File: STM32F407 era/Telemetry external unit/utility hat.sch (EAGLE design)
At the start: 4 parts, among them U1 SC18IM700IPW,112, U2 MAX1704X

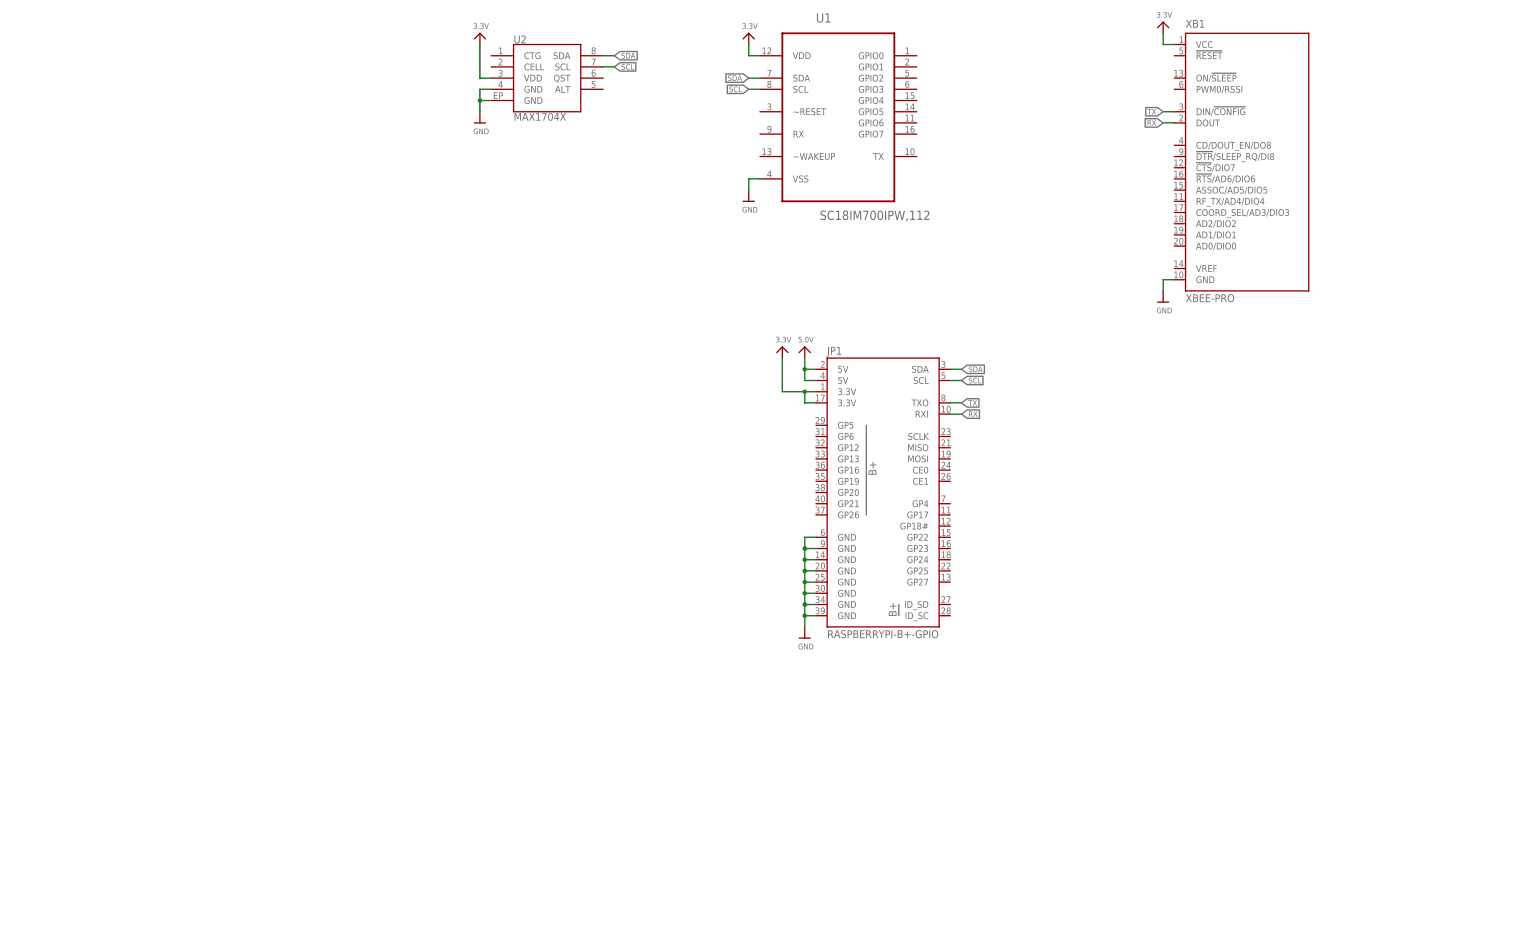
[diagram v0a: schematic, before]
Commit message: Initial Rasp Pi UPS design done
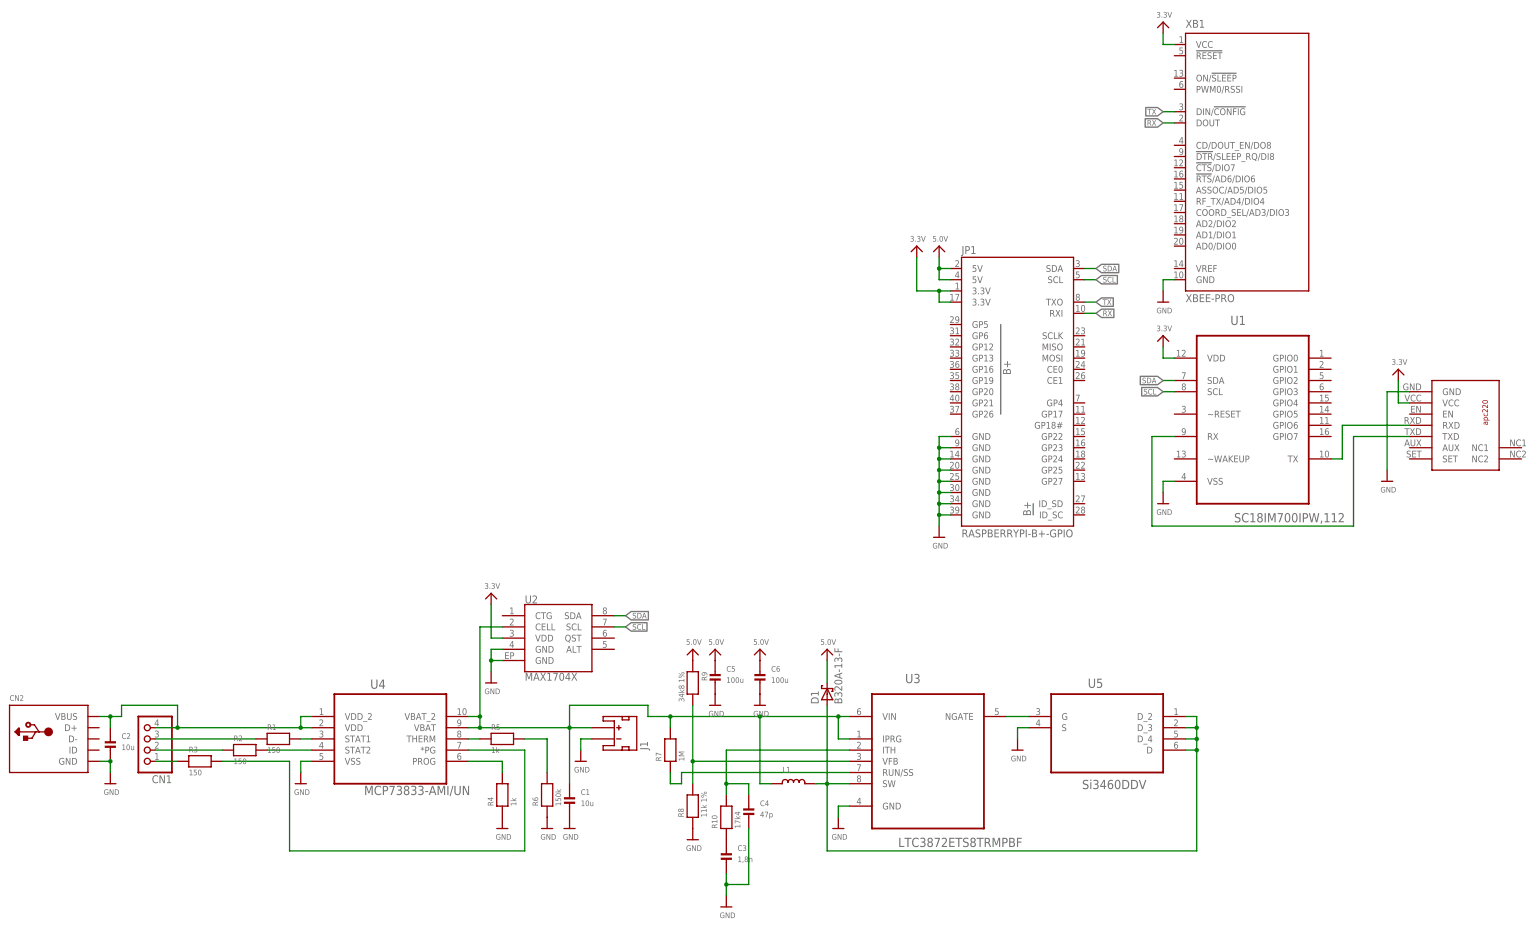
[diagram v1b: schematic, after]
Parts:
- added C1, C2: 10u, microbuilder:CAP_CERAMIC_0805MP
- added C3: 1,8n, microbuilder:CAP_CERAMIC_0603MP
- added C4: 47p, microbuilder:CAP_CERAMIC_0603MP
- added C5, C6: 100u, microbuilder:CAP_CERAMIC1206
- added CN1: (no value), microbuilder:JST_4PIN
- added CN2: (no value), adafruit:USBMINIB
- added D1: B320A-13-F, diode:MBRS320T3
- added J1: (no value), SparkFun-Connectors:JST_2MM_MALE
- added L1: (no value), microbuilder:INDUCTOR
- added R1, R2, R3: 150, microbuilder:RESISTOR_0603MP
- added R10: 17k4, microbuilder:RESISTOR_0603MP
- added R4, R5: 1k, microbuilder:RESISTOR_0603MP
- added R6: 150k, microbuilder:RESISTOR_0603MP
- added R7: 1M, microbuilder:RESISTOR_0603MP
- added R8: 11k 1%, microbuilder:RESISTOR_0603MP
- added R9: 34k8 1%, microbuilder:RESISTOR_0603MP
- added U$10: APC220, APC220:APC220
- added U3: LTC3872ETS8TRMPBF, LTC_By_element14_Batch_1:LTC3872ETS8TRMPBF
- added U4: MCP73833-AMI/UN, Microchip_By_element14_Batch_1:MCP73833-AMI/UN
- added U5: Si3460DDV, Vishay_By_element14_Batch_1:SI3457CDV-T1-GE3
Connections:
- new net N$1: U$10.RXD, U1.TX
- new net N$10: C1.P$1, J1.+, L1.1, R7.2, U2.CELL, U3.IPRG, U3.VIN, U4.VBAT, U4.VBAT_2
- new net N$11: R4.2, U4.PROG
- new net N$12: R5.1, U4.THERM
- new net N$13: R5.2, R6.2
- new net N$14: R7.1, U3.RUN/SS
- new net N$15: R8.2, R9.2, U3.VFB
- new net N$16: C4.P$1, R10.2, U3.ITH
- new net N$17: C3.P$1, R10.1
- new net N$19: D1.A, L1.2, U3.SW, U5.D, U5.D_2, U5.D_3, U5.D_4
- new net N$2: U$10.TXD, U1.RX
- new net N$21: U3.NGATE, U5.G
- new net N$3: C2.P$1, CN1.4, CN2.VBUS, U4.VDD, U4.VDD_2
- new net N$4: R1.2, U4.STAT1
- new net N$5: R2.2, U4.STAT2
- new net N$6: R3.2, U4.*PG
- new net N$7: CN1.1, R3.1
- new net N$8: CN1.2, R2.1
- new net N$9: CN1.3, R1.1
- net 3.3V: now also U$10.VCC
- net 5.0V: now also C5.P$1, C6.P$1, D1.C, R9.1
- net GND: now also C1.P$2, C2.P$2, C3.P$2, C4.P$2, C5.P$2, C6.P$2, CN2.GND, J1.-, R4.1, R6.1, R8.1, U$10.GND, U3.GND, U4.VSS, U5.S
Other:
- moved on the sheet: JP1, U1, U2
